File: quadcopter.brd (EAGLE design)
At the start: 130.1 x 130.4 mm, 78 parts, among them J1 ISP, U2 ATMEGA128RFA1

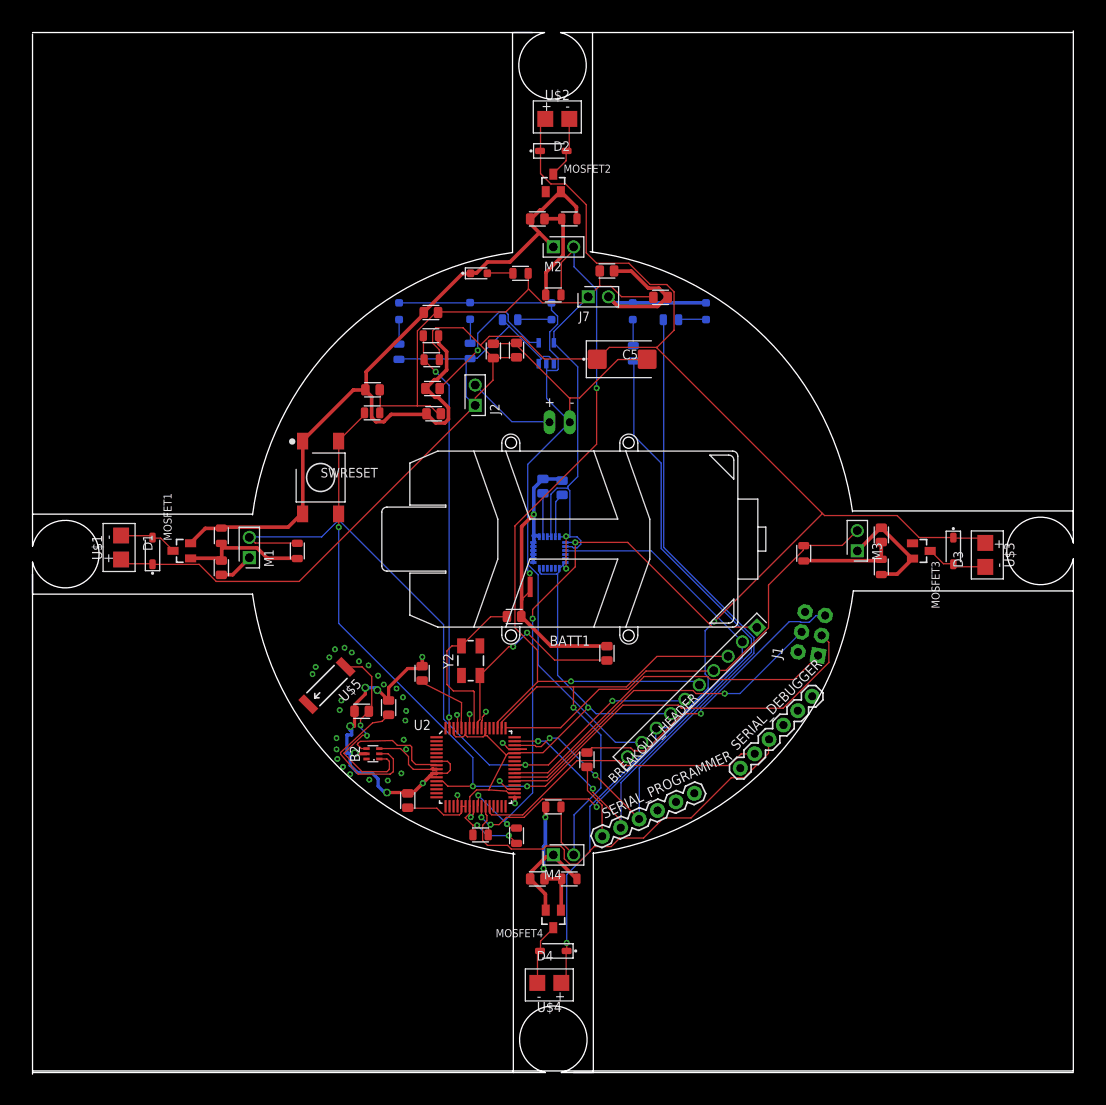
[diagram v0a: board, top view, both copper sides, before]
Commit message: After fixing professor's comments
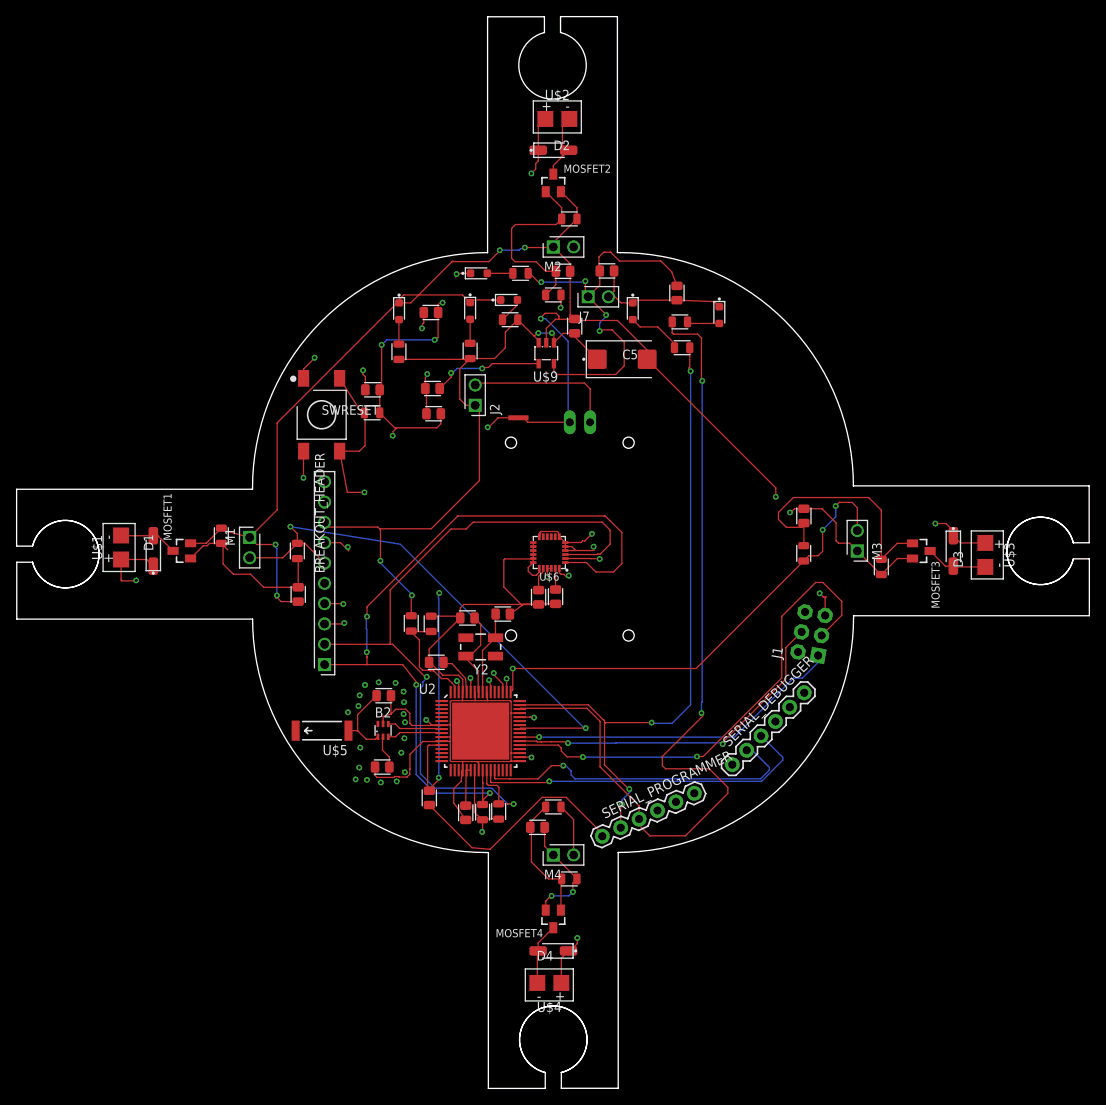
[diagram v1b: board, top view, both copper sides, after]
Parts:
- removed C7: 10uF, quadparts_prebuilt:CAPC2012X140_HS
- removed C8: 0.01uF, quadparts_prebuilt:CAPC2012X140_HS
- added C6: 0.1uF, quadparts_prebuilt:CAPC2012X140_HS
- C10, C13, C14: value 1uF -> 0.1uF
- D1, D2, D3, D4: value (none) -> 360mV
- moved C10 73.1 mm to (31.3, 4.38), turned to 90 degrees
- moved C18 69.3 mm to (2.67, 28.1), turned to 90 degrees
- moved C13 55.6 mm to (-31.9, -5.44), turned to 270 degrees
- moved BREAKOUT_HEADER 54.2 mm to (-28.6, -14.2), turned to 90 degrees
- moved C14 51.7 mm to (1.21, 35.0), turned to 0 degrees
- moved R6 36.0 mm to (-15.3, -9.11), turned to 270 degrees
- moved R5 33.1 mm to (-17.8, -9.06), turned to 90 degrees
- moved U$7 21.9 mm to (-5.00, 16.6), turned to 180 degrees
- moved C15 20.3 mm to (-15.5, -30.9)
- moved C1 13.9 mm to (-6.32, -7.89), turned to 0 degrees
- moved C21 13.9 mm to (-1.84, -5.79), flipped to the top, turned to 270 degrees
- moved C20 13.6 mm to (0.28, -5.72), flipped to the top, turned to 90 degrees
- moved SWRESET 7.84 mm to (-29.0, 17.0)
- moved C22 7.47 mm to (-21.4, -27.0), turned to 0 degrees
- moved C23 7.41 mm to (-10.9, -32.7), turned to 270 degrees
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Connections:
- removed net N$15: C13.1, R13.2, R14.2
- removed net N$20: C14.1, R15.2, R16.2
- net BAT_GND: now also C10.2, C13.2, C14.2, C18.2, C6.2, M1.1, M2.1, M3.1, M4.1, MOSFET1.2, MOSFET2.2, MOSFET3.2, MOSFET4.2, R11.1, R13.1, R15.1, R17.1; no longer C7.2, C8.2
- net GND: no longer C10.2, C13.2, C14.2, C18.2, M1.1, M2.1, M3.1, M4.1, MOSFET1.2, MOSFET2.2, MOSFET3.2, MOSFET4.2, R11.1, R13.1, R15.1, R17.1
- net N$2: now also C13.1; no longer C10.1
- net N$48: now also C14.1, R13.2, R14.2
- net N$50: now also C10.1, R15.2, R16.2
- net N$52: now also C6.1; no longer C18.1
- net VBAT: now also C18.1; no longer C7.1, C8.1
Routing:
- net BAT_GND: track 118.3 -> 295.0 mm, vias 1 -> 9
- net VBAT: track 300.1 -> 131.1 mm, vias 2 -> 8
- net GND: track 280.3 -> 192.6 mm, vias 16 -> 8
- net VBAT_SENSE: track 50.5 -> 13.7 mm, vias 2 -> 0
- net N$50: track 0.00 -> 32.6 mm
- net PWM3: track 57.7 -> 87.2 mm, vias 0 -> 4
- net N$48: track 0.00 -> 24.4 mm
- net SCL: track 74.7 -> 97.0 mm
- net PWM2: track 95.9 -> 115.5 mm
- net SDA: track 74.4 -> 93.7 mm, vias 3 -> 2
- net DTR: track 9.48 -> 28.8 mm
- net RX0: track 93.3 -> 111.3 mm
- net PWM1: track 85.8 -> 68.6 mm
- net N$4: track 26.3 -> 10.4 mm, vias 2 -> 0
- net RFANT: track 25.3 -> 9.60 mm, vias 2 -> 0
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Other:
- board size 130.1 x 130.4 mm -> 134.1 x 134 mm
